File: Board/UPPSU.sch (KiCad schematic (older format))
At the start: 48 parts, among them J1 Conn_01x04_Male, J2 ARDUINO, K1 FINDER-30.22, Q1 BC547, U1 AMSRI-7805-NZ, U2 LM324, U3 ADM2483xRW

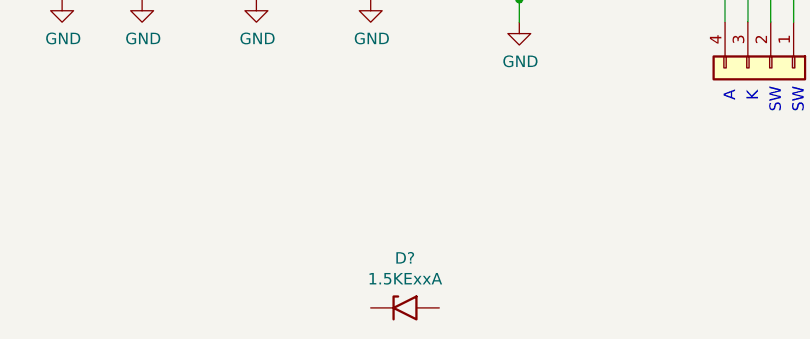
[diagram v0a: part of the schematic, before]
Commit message: Initial release
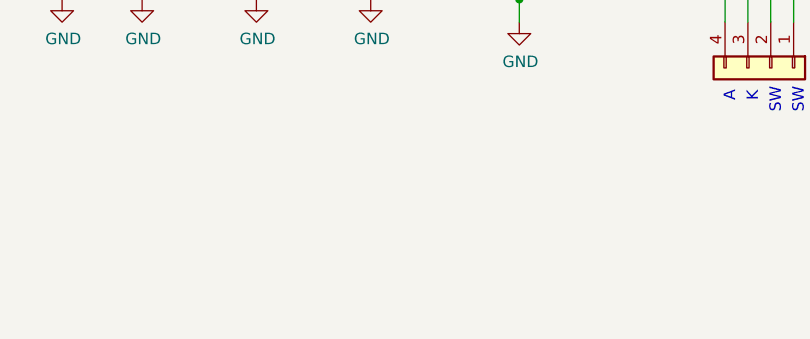
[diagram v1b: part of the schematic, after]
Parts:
- removed D?: 1.5KExxA, Diode_THT:D_DO-201AE_P15.24mm_Horizontal, symbol Diode:1.5KExxA
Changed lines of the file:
@@
 Wire Wire Line
 	8200 4500 8850 4500
-$Comp
-L Diode:1.5KExxA D?
-U 1 1 60543B6D
-P 3650 7400
-F 0 "D?" H 3650 7617 50  0000 C CNN
-F 1 "1.5KExxA" H 3650 7526 50  0000 C CNN
-F 2 "Diode_THT:D_DO-201AE_P15.24mm_Horizontal" H 3650 7200 50  0001 C CNN
-F 3 "https://www.vishay.com/docs/88301/15ke.pdf" H 3600 7400 50  0001 C CNN
-	1    3650 7400
-	1    0    0    -1
-$EndComp
 $EndSCHEMATC

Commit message: test
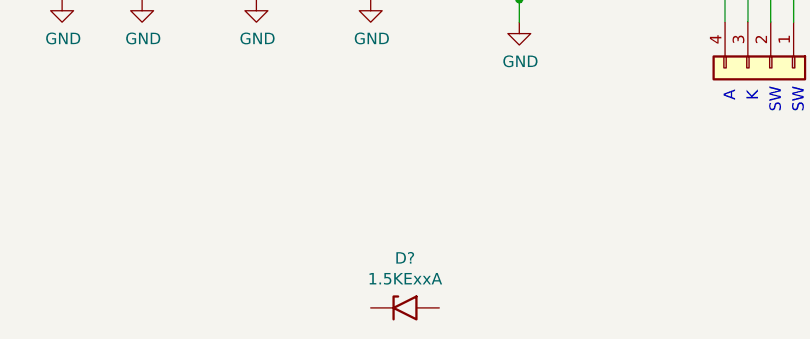
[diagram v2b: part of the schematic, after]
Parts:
- added D?: 1.5KExxA, Diode_THT:D_DO-201AE_P15.24mm_Horizontal, symbol Diode:1.5KExxA
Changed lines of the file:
@@
 Wire Wire Line
 	8200 4500 8850 4500
+$Comp
+L Diode:1.5KExxA D?
+U 1 1 60543B6D
+P 3650 7400
+F 0 "D?" H 3650 7617 50  0000 C CNN
+F 1 "1.5KExxA" H 3650 7526 50  0000 C CNN
+F 2 "Diode_THT:D_DO-201AE_P15.24mm_Horizontal" H 3650 7200 50  0001 C CNN
+F 3 "https://www.vishay.com/docs/88301/15ke.pdf" H 3600 7400 50  0001 C CNN
+	1    3650 7400
+	1    0    0    -1
+$EndComp
 $EndSCHEMATC
